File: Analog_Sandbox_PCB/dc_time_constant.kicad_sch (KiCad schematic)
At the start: 14 parts, among them J21 PAD, Q2 PAD, U2 NE555P

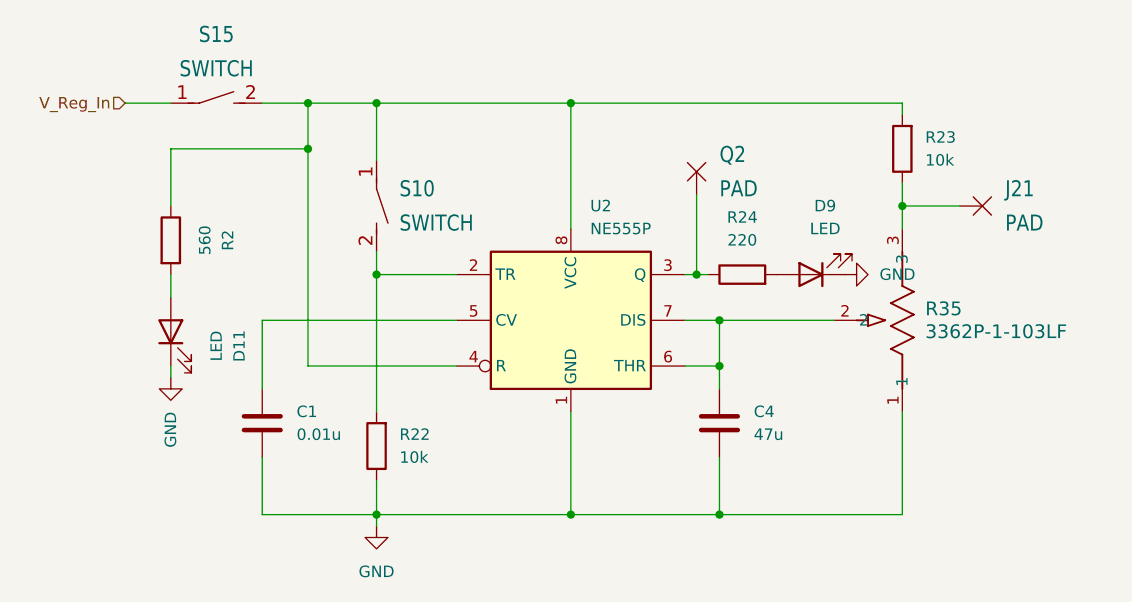
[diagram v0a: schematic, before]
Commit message: made changes from morning of 4/13
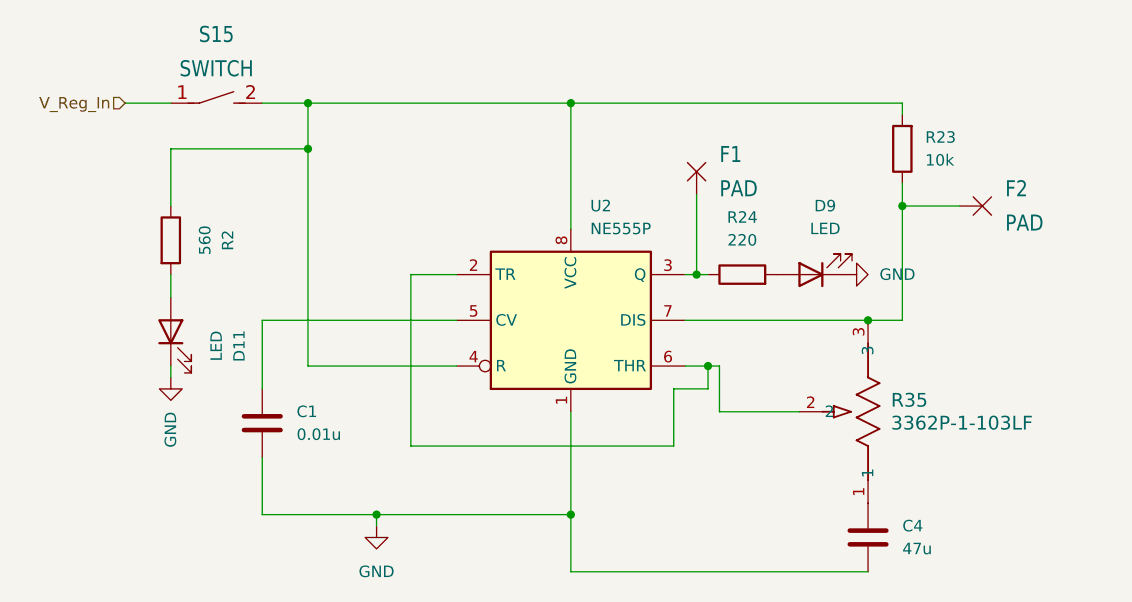
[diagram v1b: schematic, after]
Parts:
- removed R22: 10k, Resistor_SMD:R_1206_3216Metric, symbol Device:R
- removed S10: SWITCH, Button_Switch_THT:SW_DIP_SPSTx01_Slide_9.78x4.72mm_W7.62mm_P2.54mm, symbol Analog_Sandbox_PCB-eagle-import:DS01E
- renumbered Q2 to F1, J21 to F2
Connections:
- net GND: no longer R35.1
- net at F2.1 (P), R23.1, R35.3: now also U2.7 (DIS)
- net at R35.2, U2.6 (THR): now also U2.2 (TR); no longer C4.1, U2.7 (DIS)
- new net: C4.1, R35.1
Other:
- moved on the sheet: C4, R35
